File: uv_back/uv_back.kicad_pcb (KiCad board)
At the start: 2 copper layers, 75 x 174.2 mm, 0 parts

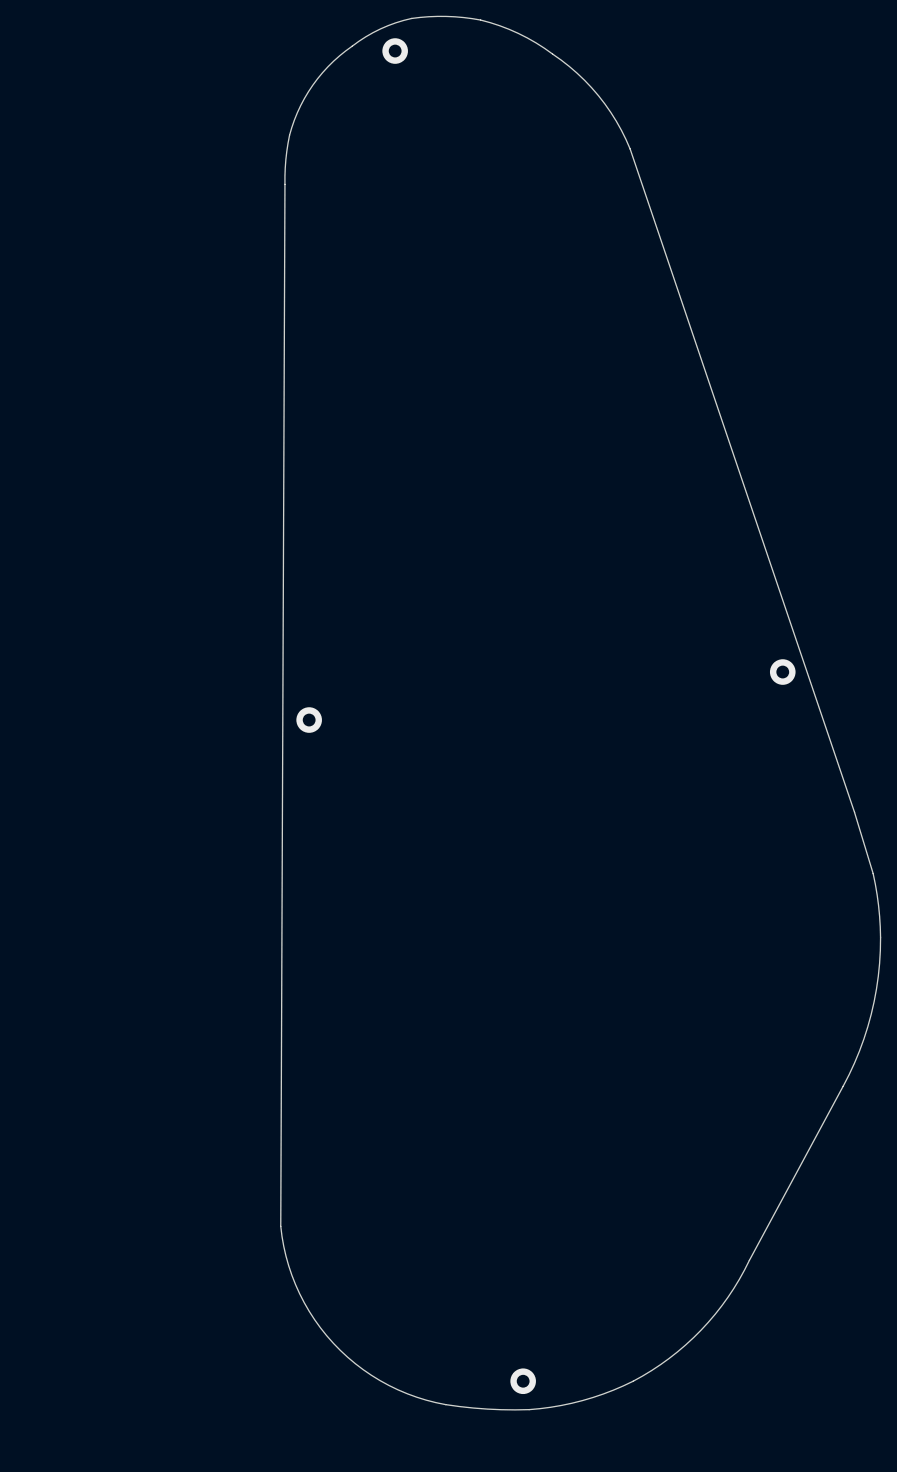
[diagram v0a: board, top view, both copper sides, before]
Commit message: setting up for KiCad v6.01
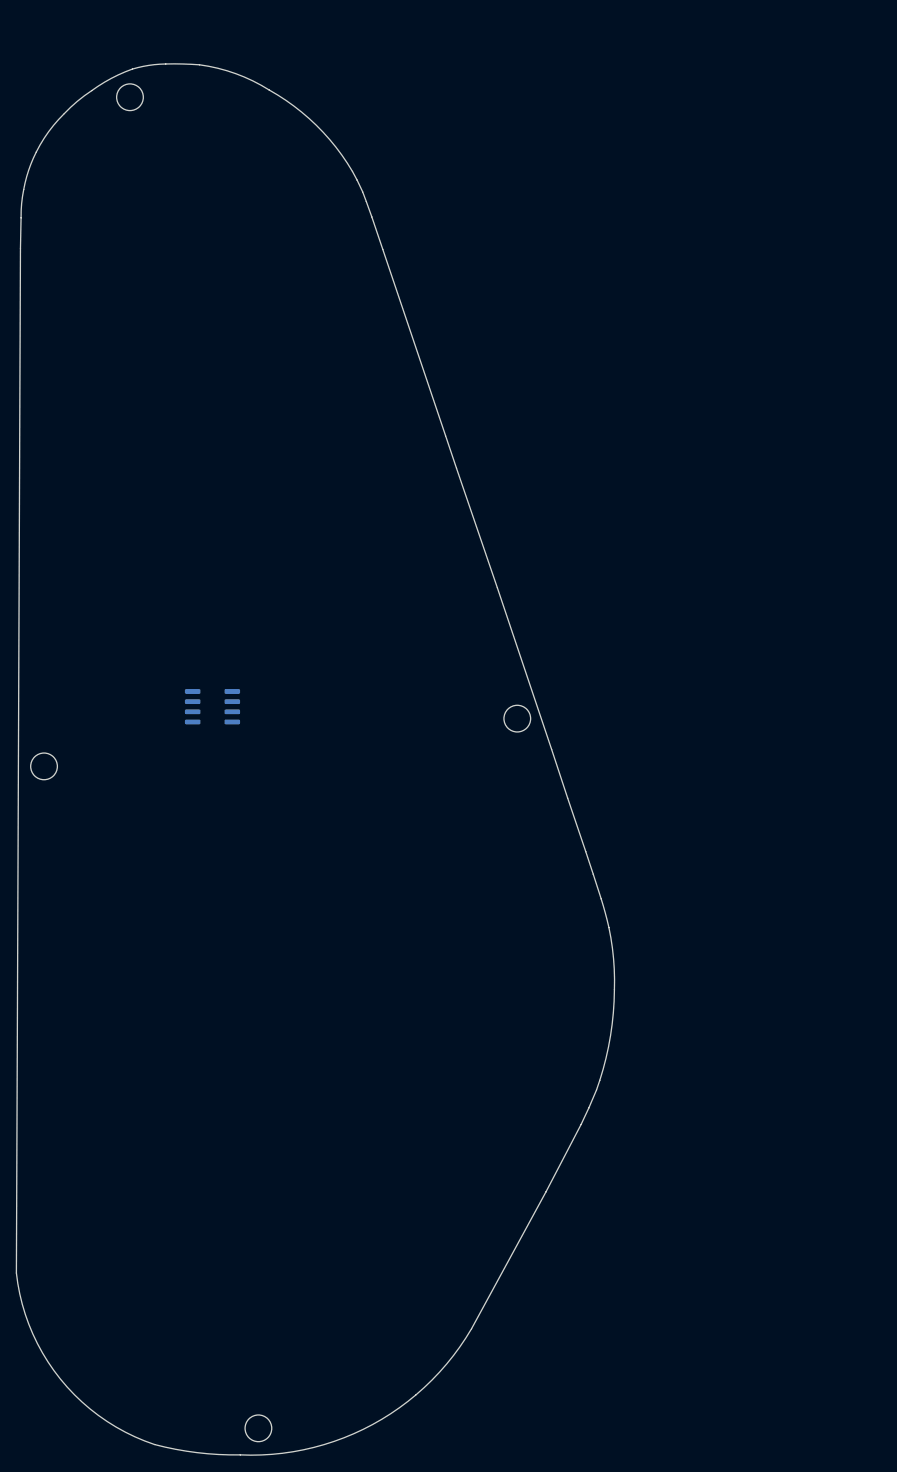
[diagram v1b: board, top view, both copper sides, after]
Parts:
- added U1: OPA1656ID, Package_SO:SOIC-8_3.9x4.9mm_P1.27mm, B.Cu at (67.6, 102.2)
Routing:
- net (no net): vias 4 -> 0
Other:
- board size 75 x 174.2 mm -> 74.8 x 173.9 mm
